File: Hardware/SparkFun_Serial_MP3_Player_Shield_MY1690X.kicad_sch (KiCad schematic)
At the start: 42 parts, among them J1 3.5mm TRRS, J2 Conn_01x04, J4 USB_C_Receptacle, J6 microSD, Q1 BSS138, SW1 SMD_5.2x5.2mm_h2.5mm, U2 MY1690X

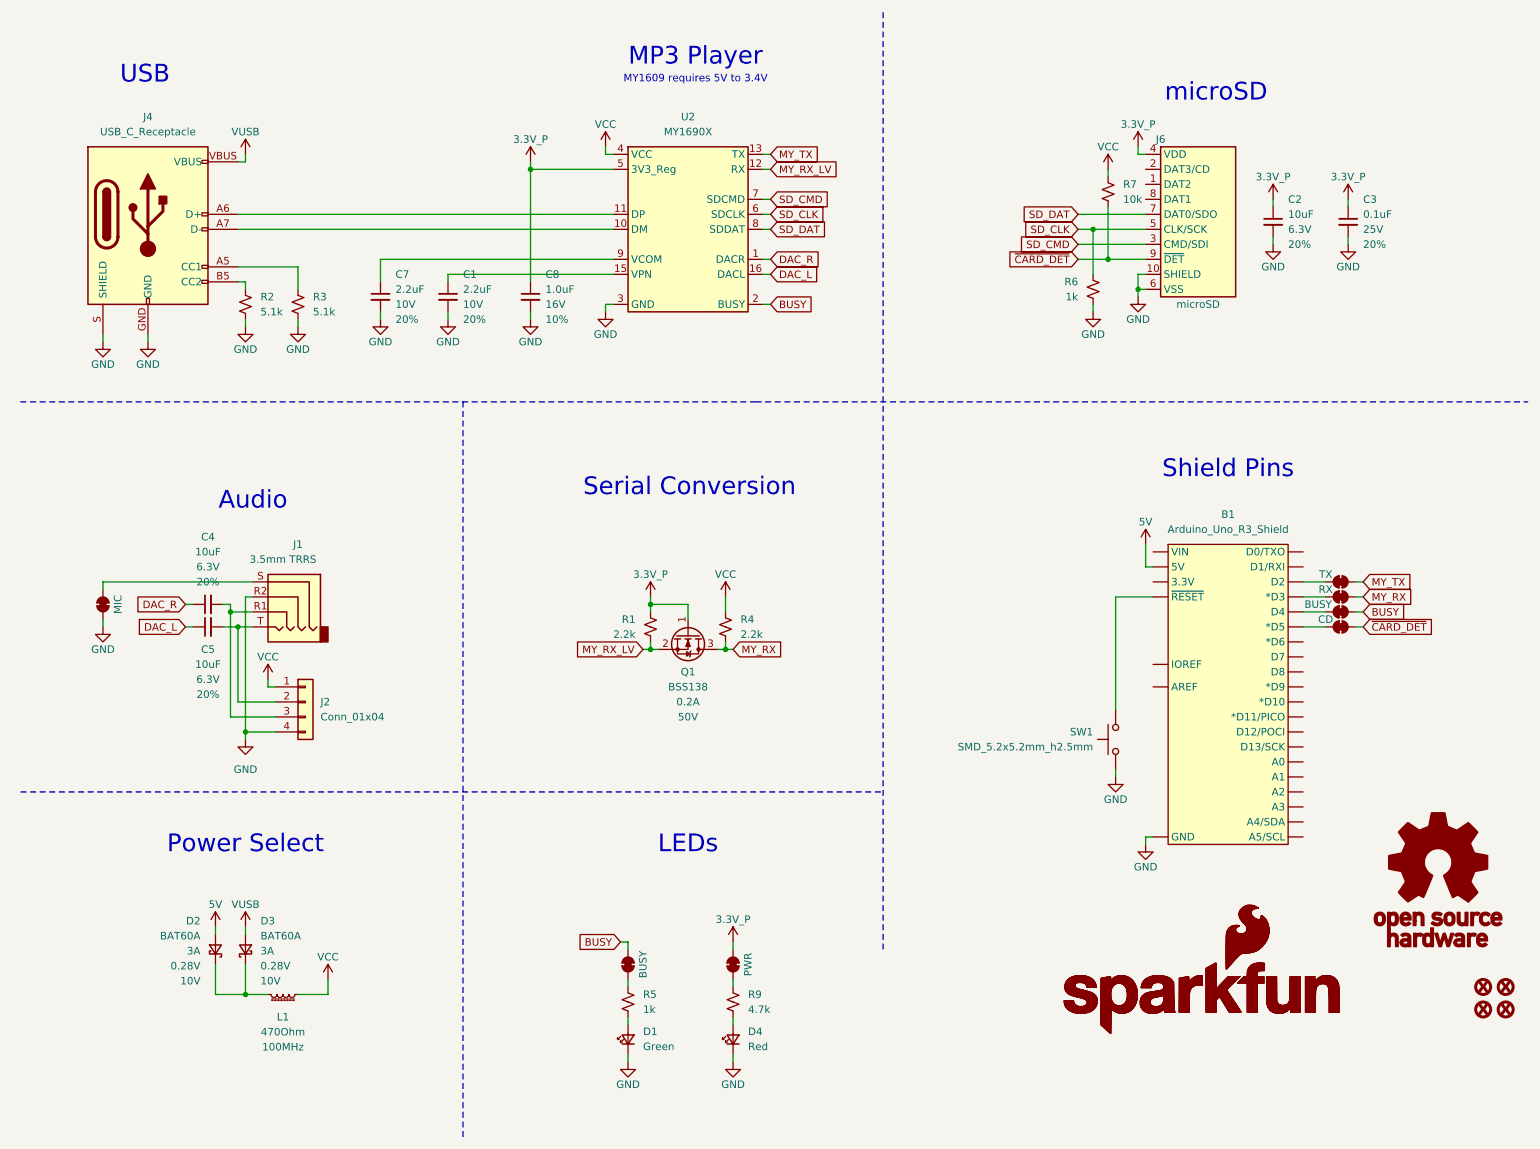
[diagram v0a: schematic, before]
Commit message: Post review updates.
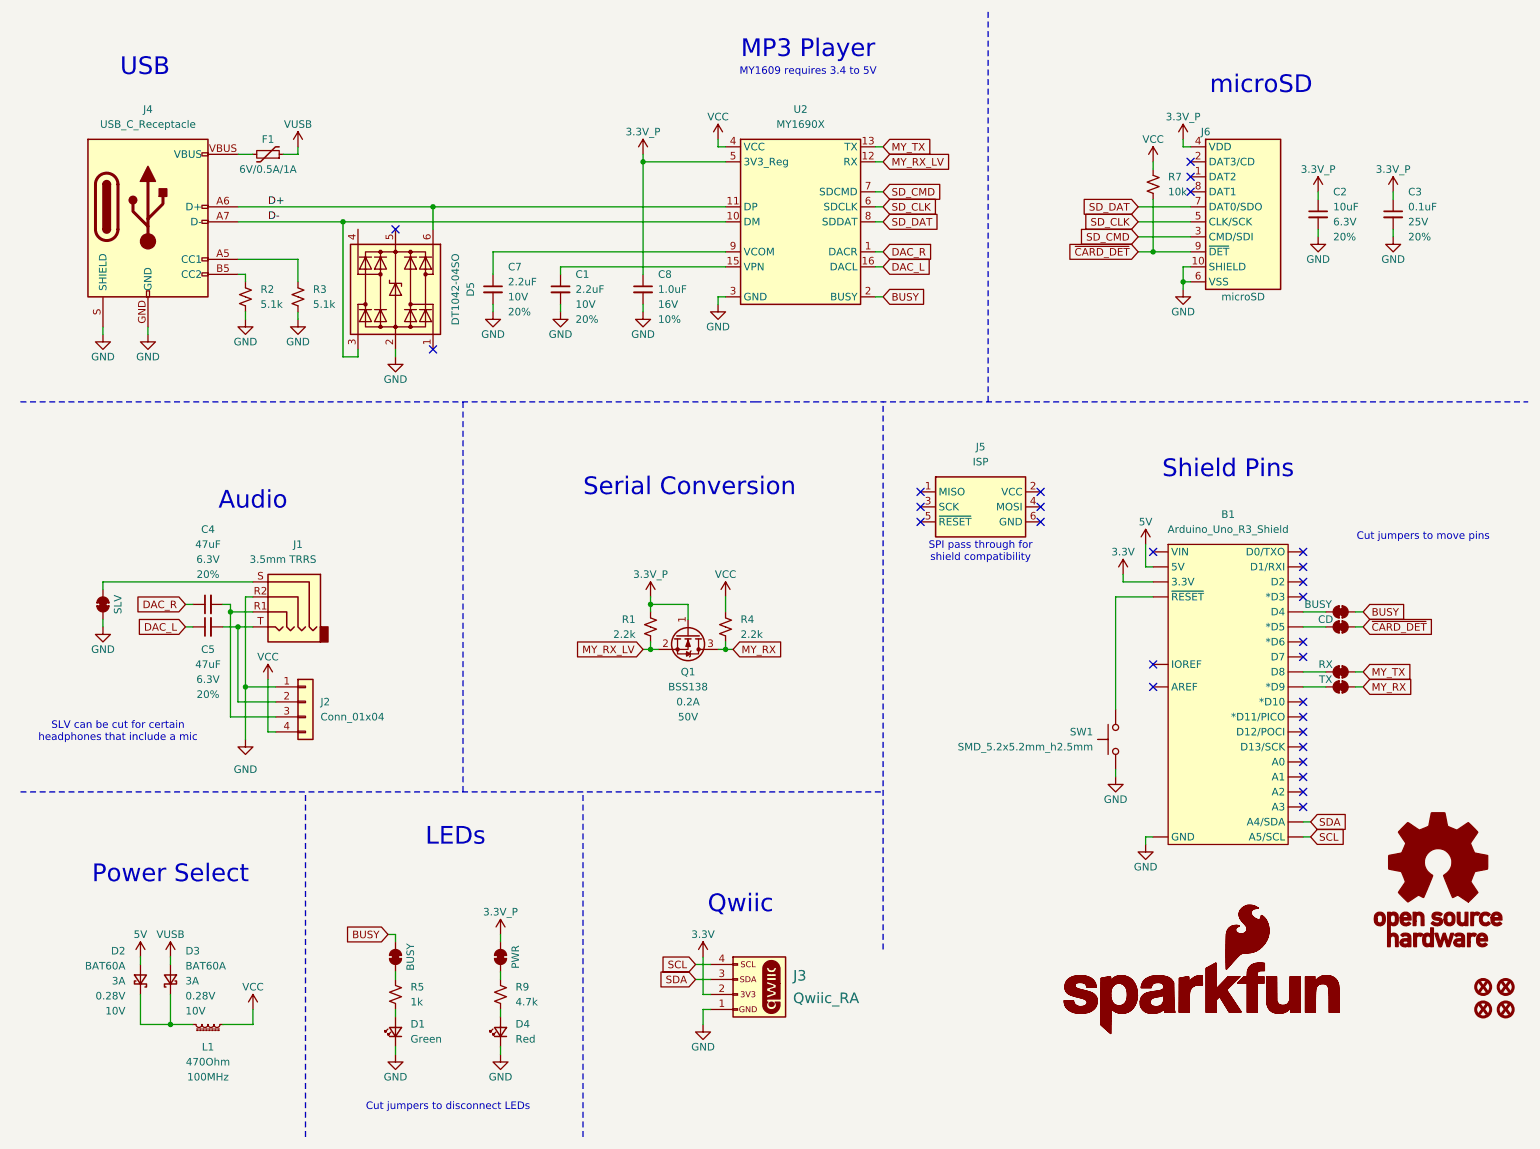
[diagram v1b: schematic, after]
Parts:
- removed R6: 1k, SparkFun-Resistor:R_0603_1608Metric, symbol SparkFun-Resistor:1k_0603
- added D5: DT1042-04SO, SparkFun-Semiconductor-Standard:SOT23-6, symbol SparkFun-DiscreteSemi:D_TVS_ESD_USB
- added F1: 6V/0.5A/1A, SparkFun-Fuse:0805, symbol SparkFun-Fuse:Fuse 6V/0.5A/1A
- added J3: Qwiic_RA, SparkFun-Connector:JST_SMD_1.0mm-4_Black, symbol SparkFun-Connector:Qwiic_Right_Angle
- added J5: ISP, SparkFun-Connector:2x03_NoSilk, symbol SparkFun-Connector:AVR_ISP_PTH
- C4, C5: value 10uF -> 47uF; footprint SparkFun-Capacitor:C_0603_1608Metric -> SparkFun-Capacitor:C_0805_2012Metric; symbol SparkFun-Capacitor:10uF_0603_6.3V_20% -> SparkFun-Capacitor:47uF_0805_6.3V_20%; PROD_ID CAP-11015 -> CAP-13854
- JP7: value MIC -> SLV
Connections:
- net GND: now also J2.1 (Pin_1), D5.2 (GND), J3.1 (Pin_1); no longer J2.4 (Pin_4)
- net MY_RX: now also JP6.2 (B); no longer JP5.2 (B)
- net MY_TX: now also JP5.2 (B); no longer JP6.2 (B)
- net VCC: now also J2.4 (Pin_4); no longer J2.1 (Pin_1)
- net VUSB: now also F1.1; no longer J4.VBUS
- net D+: now reaches J4.A6 (D+), J4.B6 (D+), U2.11 (DP)
- net D+: now also D5.6 (I/O4)
- net D-: now reaches J4.A7 (D-), J4.B7 (D-), U2.10 (DM)
- net D-: now also D5.3 (I/O2)
- net at JP5.1 (A): now also B1.D8; no longer B1.D3 (*D3)
- net 3.3V: now reaches B1.3.3V
- net 3.3V: now also J3.2 (Pin_2)
- net SDA: now reaches B1.A4/SDA
- net SDA: now also J3.3 (Pin_3)
- net SCL: now reaches B1.A5/SCL
- net SCL: now also J3.4 (Pin_4)
- net at JP6.1 (A): now also B1.D9 (*D9); no longer B1.D2
- new net: F1.2, J4.VBUS
- no-connect marks 0 -> 28
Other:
- note added: "Cut jumpers to disconnect LEDs"
- note added: "Cut jumpers to move pins"
- note added: "MY1609 requires 3.4 to 5V"
- note added: "Qwiic"
- note added: "SLV can be cut for certain headphones that include a mic"
- note added: "SPI pass through for shield compatibility"
- note removed: "MY1609 requires 5V to 3.4V"
- moved on the sheet: C1, C2, C3, C7, C8, D1, D2, D3, D4, J4, J6, L1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
